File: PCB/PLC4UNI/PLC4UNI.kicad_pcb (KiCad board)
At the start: 4 copper layers, 102.4 x 83.1 mm, 209 parts, among them J1 Conn_02x08_Odd_Even, K1 G5V-1-DC3, K2 G5V-1-DC3, Q1 ZXMS6004FFQTA, Q2 ZXMS6004FFQTA, Q3 ZXMS6004FFQTA, Q4 ZXMS6004FFQTA, Q5 NCE60P04R, SW1 TS-1088-AR02016, SW2 TS-1088-AR02016, U1 ScrewTerminal1-1x9-P5.0mm, U10 AT3H4B-CUH-S, U11 AT3H4B-CUH-S, U12 AT3H4B-CUH-S, U13 AT3H4B-CUH-S, U14 AT3H4B-CUH-S, U15 MAX31856MUD+, U16 GP8211S-TC50-EW, U17 GP8302-TC50-EW, U18 BL0942, U19 B0303S-1WR3_C7465185, U2 ScrewTerminal1-1x9-P5.0mm, U20 ISO7021DR, U21 AP63203WU-7, U22 APH0630T4R7M, U23 TD301M485_C5451847, U3 ScrewTerminal1-1x9-P5.0mm, U4 ScrewTerminal1-1x9-P5.0mm, U5 ADS1115IDGS, U6 ESP32-S3-WROOM-1, U7 BTS723GWXUMA1, U8 LK1802, U9 AT3H4B-CUH-S

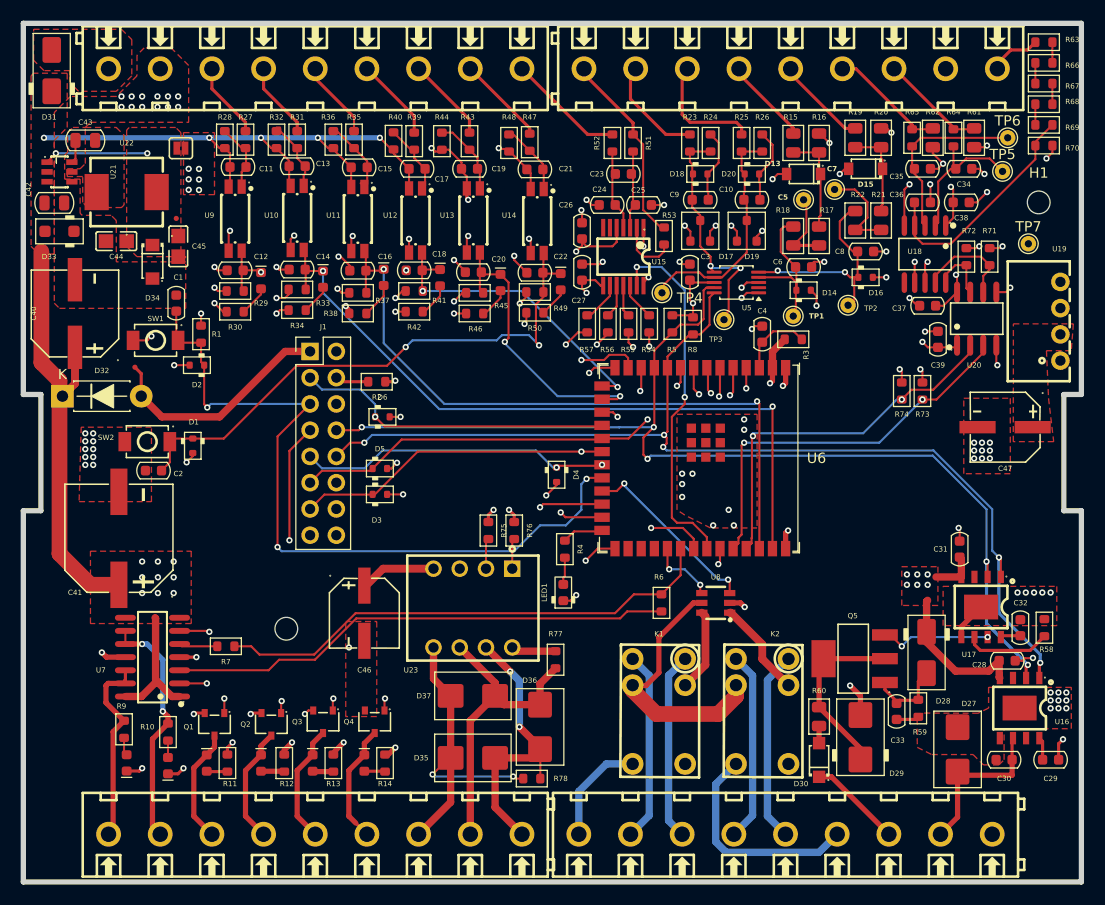
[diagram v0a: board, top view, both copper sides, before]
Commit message: ensamblado en proceso
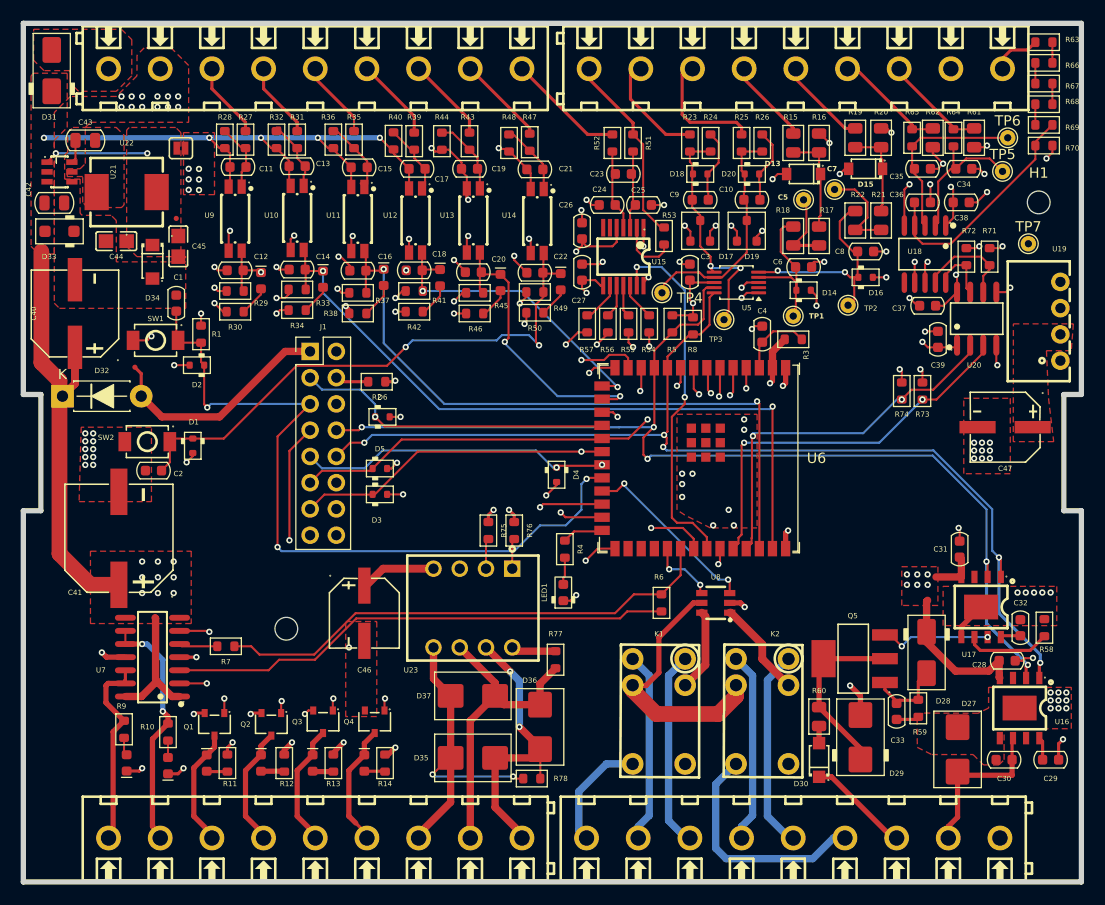
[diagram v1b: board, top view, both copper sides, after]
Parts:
- moved U4 0.83 mm to (228.4, 163.4)
- moved U2 0.50 mm to (228.7, 89.0)
- moved U3 0.37 mm to (182.2, 163.4)
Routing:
- net /plc4uni_top/CON_OUT_RLY2-COM: track 21.3 -> 22.7 mm
- net /plc4uni_top/CON_OUT_RLY1-NO: track 18.2 -> 19.1 mm
- net /plc4uni_top/CON_OUT_4-20MA_1: track 9.05 -> 9.95 mm
- net /plc4uni_top/CON_OUT_RLY2-NO: track 18.5 -> 19.4 mm
- net /plc4uni_top/CON_OUT_RLY1-COM: track 10.5 -> 11.1 mm
- net /plc4uni_top/CON_IN_0-10V_1: track 10.3 -> 10.8 mm
- net /plc4uni_top/CON_IN_0-10V_2: track 11.6 -> 12.1 mm
